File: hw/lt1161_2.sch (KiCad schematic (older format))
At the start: 7 parts, among them U601 VND5050AJTR-E, U602 BTS6133D, U603 BTS6133D

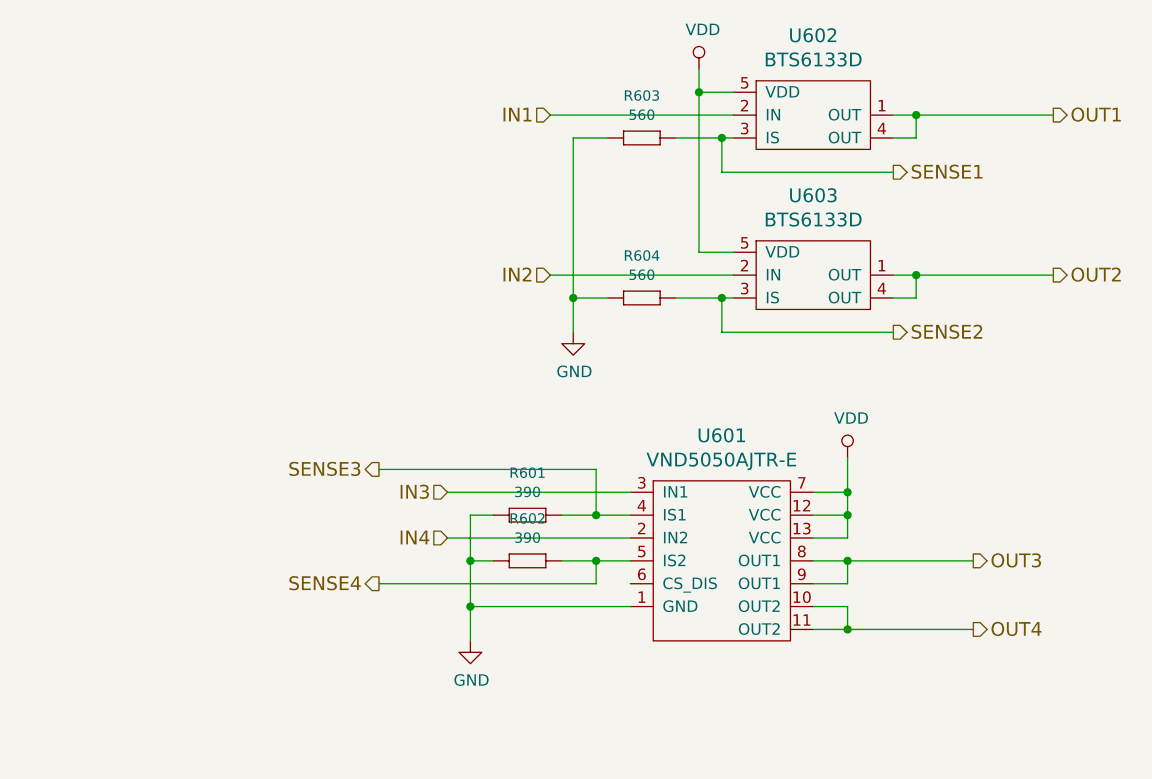
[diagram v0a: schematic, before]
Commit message: 4.1.0 hw created, not yet ordered
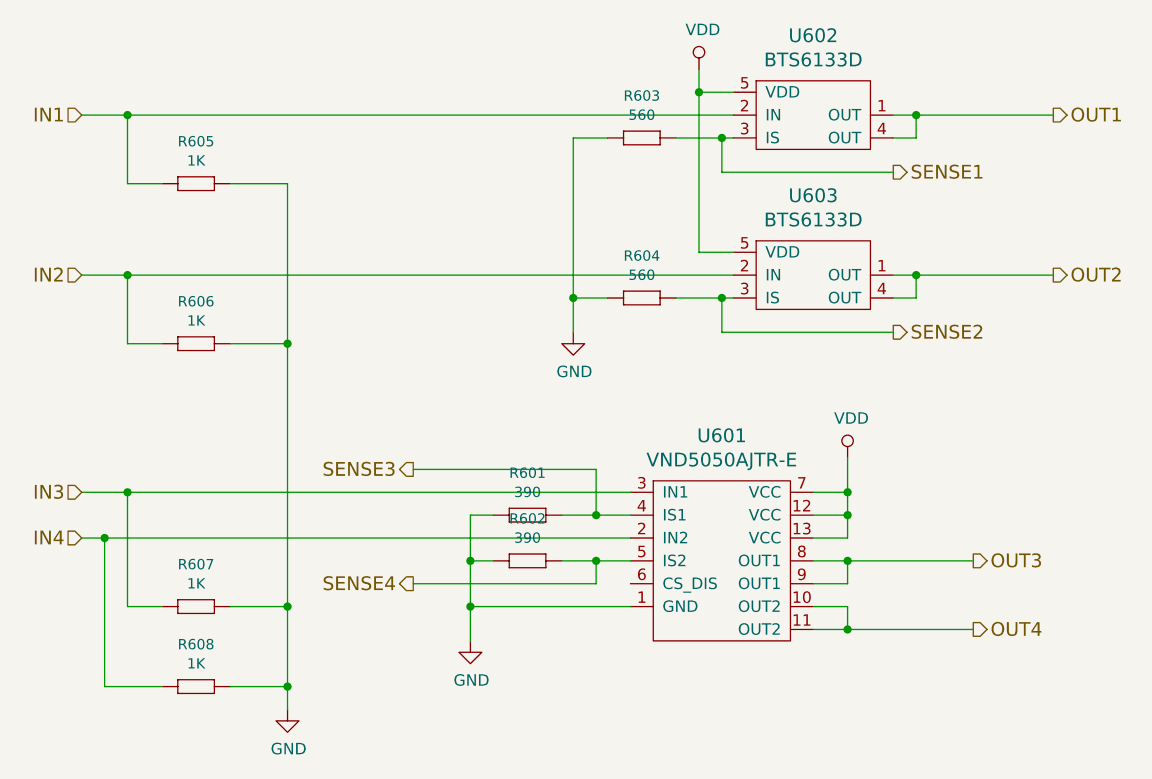
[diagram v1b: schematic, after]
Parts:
- added R605, R606, R607, R608: 1K, yageo:0603, symbol 1K
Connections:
- net GND: now also R605.1 (R1), R606.1 (R1), R607.1 (R1), R608.1 (R1)
- net IN1: now also R605.2 (R2)
- net IN2: now also R606.2 (R2)
- net IN3: now also R607.2 (R2)
- net IN4: now also R608.2 (R2)
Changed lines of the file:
@@
 Text HLabel 5800 4400 2    60   Output ~ 0
 OUT4
-Text HLabel 3950 2150 0    60   Input ~ 0
+Text HLabel 1900 2150 0    60   Input ~ 0
 IN1
-Text HLabel 3950 2850 0    60   Input ~ 0
+Text HLabel 1900 2850 0    60   Input ~ 0
 IN2
-Text HLabel 3500 3800 0    60   Input ~ 0
+Text HLabel 1900 3800 0    60   Input ~ 0
 IN3
-Text HLabel 3500 4000 0    60   Input ~ 0
+Text HLabel 1900 4000 0    60   Input ~ 0
 IN4
 Text HLabel 5450 2400 2    60   Output ~ 0
@@
 Text HLabel 5450 3100 2    60   Output ~ 0
 SENSE2
-Text HLabel 3200 3700 0    60   Output ~ 0
+Text HLabel 3350 3700 0    60   Output ~ 0
 SENSE3
-Text HLabel 3200 4200 0    60   Output ~ 0
+Text HLabel 3350 4200 0    60   Output ~ 0
 SENSE4
 $Comp
@@
 $EndComp
 $Comp
-L VDD #PWR025
+L VDD #PWR605
 U 1 1 59D808C7
 P 5250 3650
-F 0 "#PWR025" H 5250 3500 50  0001 C CNN
+F 0 "#PWR605" H 5250 3500 50  0001 C CNN
 F 1 "VDD" H 5267 3823 50  0000 C CNN
 F 2 "" H 5250 3650 50  0000 C CNN
@@
 Connection ~ 5250 4400
 Wire Wire Line
-	3500 3800 4300 3800
-Wire Wire Line
-	4300 4000 3500 4000
-$Comp
-L GND #PWR026
+	1900 3800 4300 3800
+Wire Wire Line
+	1900 4000 4300 4000
+$Comp
+L GND #PWR602
 U 1 1 59D86DC2
 P 3600 4450
-F 0 "#PWR026" H 3600 4200 50  0001 C CNN
+F 0 "#PWR602" H 3600 4200 50  0001 C CNN
 F 1 "GND" H 3605 4277 50  0000 C CNN
 F 2 "" H 3600 4450 50  0000 C CNN
@@
 	4000 3900 4300 3900
 Wire Wire Line
-	3200 4200 4150 4200
+	3350 4200 4150 4200
 Wire Wire Line
 	4150 4200 4150 4100
@@
 	4150 3900 4150 3700
 Wire Wire Line
-	4150 3700 3200 3700
+	4150 3700 3350 3700
 Connection ~ 4150 3900
 $Comp
@@
 $EndComp
 $Comp
-L VDD #PWR027
+L VDD #PWR604
 U 1 1 59D89B9B
 P 4600 1950
-F 0 "#PWR027" H 4600 1800 50  0001 C CNN
+F 0 "#PWR604" H 4600 1800 50  0001 C CNN
 F 1 "VDD" H 4617 2123 50  0000 C CNN
 F 2 "" H 4600 1950 50  0000 C CNN
@@
 Connection ~ 4700 2950
 Wire Wire Line
-	3950 2850 4750 2850
-Wire Wire Line
-	4750 2150 3950 2150
-$Comp
-L GND #PWR028
+	1900 2850 4750 2850
+Wire Wire Line
+	1900 2150 4750 2150
+$Comp
+L GND #PWR603
 U 1 1 59D8A4D0
 P 4050 3100
-F 0 "#PWR028" H 4050 2850 50  0001 C CNN
+F 0 "#PWR603" H 4050 2850 50  0001 C CNN
 F 1 "GND" H 4055 2927 50  0000 C CNN
 F 2 "" H 4050 3100 50  0000 C CNN
@@
 	5550 2250 5550 2150
 Connection ~ 5550 2150
+Wire Wire Line
+	2250 4300 2100 4300
+Wire Wire Line
+	2100 4300 2100 3800
+Connection ~ 2100 3800
+Wire Wire Line
+	2250 4650 2000 4650
+Wire Wire Line
+	2000 4650 2000 4000
+Connection ~ 2000 4000
+Wire Wire Line
+	2250 3150 2100 3150
+Wire Wire Line
+	2100 3150 2100 2850
+Connection ~ 2100 2850
+Wire Wire Line
+	2250 2450 2100 2450
+Wire Wire Line
+	2100 2450 2100 2150
+Connection ~ 2100 2150
+$Comp
+L GND #PWR601
+U 1 1 5A024814
+P 2800 4750
+F 0 "#PWR601" H 2800 4500 50  0001 C CNN
+F 1 "GND" H 2805 4577 50  0000 C CNN
+F 2 "" H 2800 4750 50  0000 C CNN
+F 3 "" H 2800 4750 50  0000 C CNN
+	1    2800 4750
+	1    0    0    -1
+$EndComp
+Wire Wire Line
+	2800 2450 2800 4750
+Wire Wire Line
+	2800 4650 2550 4650
+Wire Wire Line
+	2800 4300 2550 4300
+Connection ~ 2800 4650
+Wire Wire Line
+	2800 3150 2550 3150
+Connection ~ 2800 4300
+Wire Wire Line
+	2800 2450 2550 2450
+Connection ~ 2800 3150
+$Comp
+L 1K R605
+U 1 1 5A02ED15
+P 2350 2450
+F 0 "R605" H 2400 2634 45  0000 C CNN
+F 1 "1K" H 2400 2550 45  0000 C CNN
+F 2 "yageo:0603" H 2380 2600 20  0001 C CNN
+F 3 "" H 2319 2489 60  0001 C CNN
+F 4 "" H 2719 2889 60  0001 C CNN "1st Source Part Number"
+F 5 "Digikey" H 2619 2789 60  0001 C CNN "1st Source"
+F 6 "RC0603FR-071KL" H 2519 2689 60  0001 C CNN "Manufacturer Part Number"
+F 7 "YAGEO" H 2419 2589 60  0001 C CNN "Manufacturer"
+	1    2350 2450
+	1    0    0    -1
+$EndComp
+$Comp
+L 1K R606
+U 1 1 5A02ED9F
+P 2350 3150
+F 0 "R606" H 2400 3334 45  0000 C CNN
+F 1 "1K" H 2400 3250 45  0000 C CNN
+F 2 "yageo:0603" H 2380 3300 20  0001 C CNN
+F 3 "" H 2319 3189 60  0001 C CNN
+F 4 "" H 2719 3589 60  0001 C CNN "1st Source Part Number"
+F 5 "Digikey" H 2619 3489 60  0001 C CNN "1st Source"
+F 6 "RC0603FR-071KL" H 2519 3389 60  0001 C CNN "Manufacturer Part Number"
+F 7 "YAGEO" H 2419 3289 60  0001 C CNN "Manufacturer"
+	1    2350 3150
+	1    0    0    -1
+$EndComp
+$Comp
+L 1K R607
+U 1 1 5A02EDEA
+P 2350 4300
+F 0 "R607" H 2400 4484 45  0000 C CNN
+F 1 "1K" H 2400 4400 45  0000 C CNN
+F 2 "yageo:0603" H 2380 4450 20  0001 C CNN
+F 3 "" H 2319 4339 60  0001 C CNN
+F 4 "" H 2719 4739 60  0001 C CNN "1st Source Part Number"
+F 5 "Digikey" H 2619 4639 60  0001 C CNN "1st Source"
+F 6 "RC0603FR-071KL" H 2519 4539 60  0001 C CNN "Manufacturer Part Number"
+F 7 "YAGEO" H 2419 4439 60  0001 C CNN "Manufacturer"
+	1    2350 4300
+	1    0    0    -1
+$EndComp
+$Comp
+L 1K R608
+U 1 1 5A02EE4E
+P 2350 4650
+F 0 "R608" H 2400 4834 45  0000 C CNN
+F 1 "1K" H 2400 4750 45  0000 C CNN
+F 2 "yageo:0603" H 2380 4800 20  0001 C CNN
+F 3 "" H 2319 4689 60  0001 C CNN
+F 4 "" H 2719 5089 60  0001 C CNN "1st Source Part Number"
+F 5 "Digikey" H 2619 4989 60  0001 C CNN "1st Source"
+F 6 "RC0603FR-071KL" H 2519 4889 60  0001 C CNN "Manufacturer Part Number"
+F 7 "YAGEO" H 2419 4789 60  0001 C CNN "Manufacturer"
+	1    2350 4650
+	1    0    0    -1
+$EndComp
 $EndSCHEMATC
